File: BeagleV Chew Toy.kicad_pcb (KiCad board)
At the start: 2 copper layers, 57.2 x 51.7 mm, 147 parts, among them J1 Conn_02x05_Counter_Clockwise, J2 Conn_02x05_Counter_Clockwise, J3 Conn_02x05_Counter_Clockwise, U1 74HC245, U2 74HC245, U3 74HC245, U4 74HC245

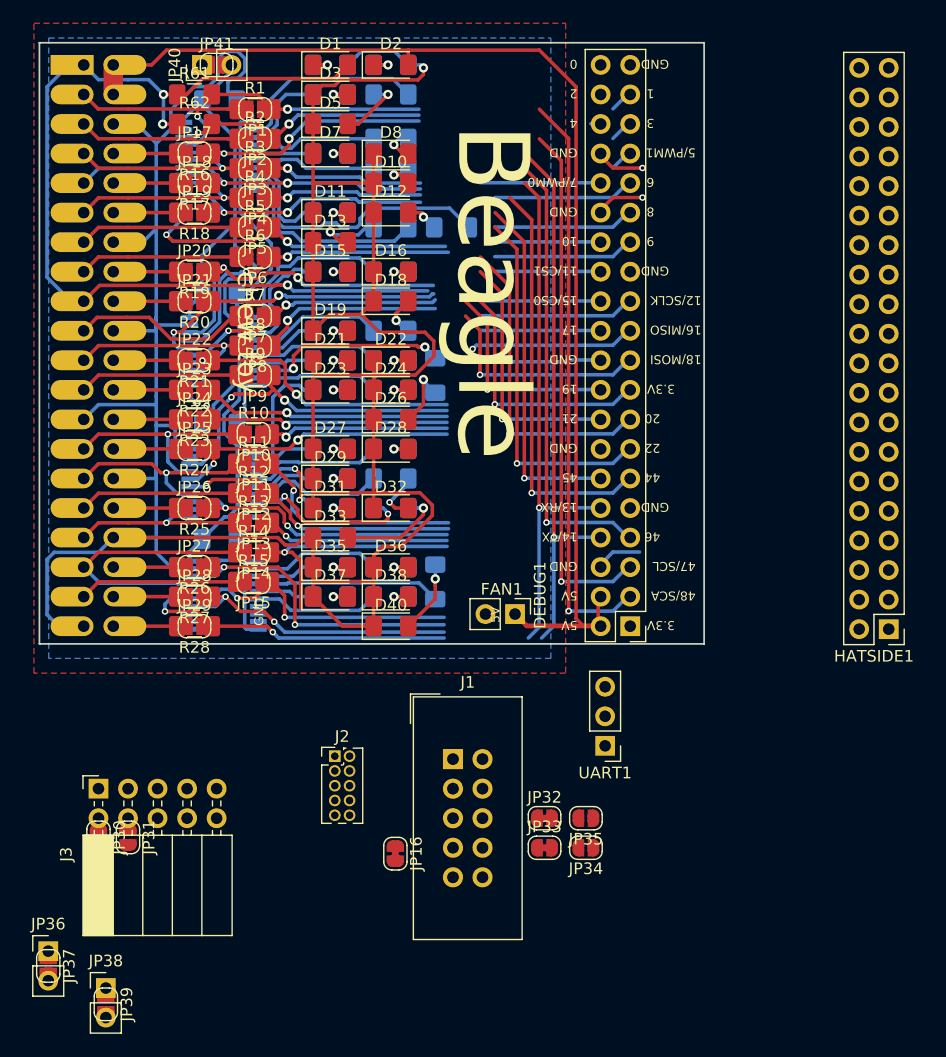
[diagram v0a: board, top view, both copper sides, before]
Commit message: main part of the PCB is done
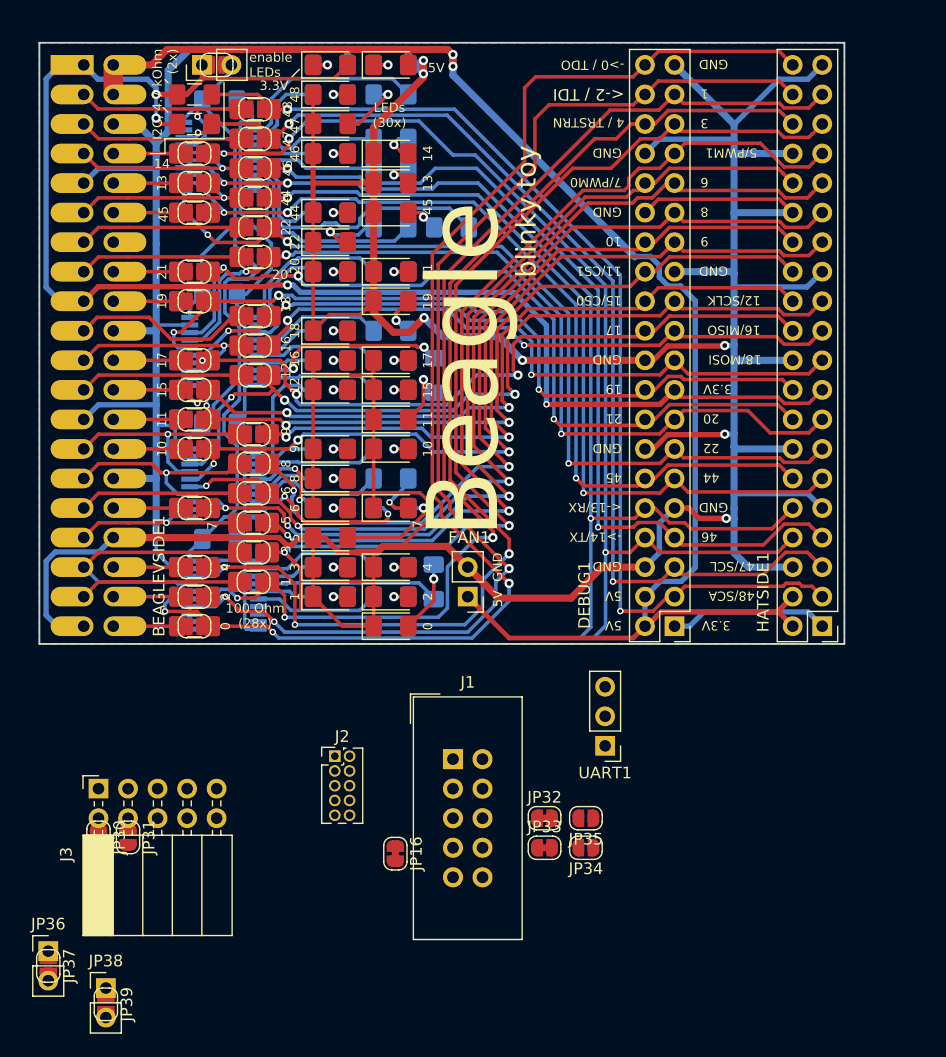
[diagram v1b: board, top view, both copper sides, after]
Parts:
- moved HATSIDE1 5.72 mm to (193.2, 129.0)
- moved FAN1 4.33 mm to (162.7, 126.5), turned to 180 degrees
- moved DEBUG1 3.81 mm to (180.5, 129.0)
- moved R32 0.13 mm to (159.8, 125.2)
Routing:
- net GND: track 359.5 -> 557.6 mm, vias 3 -> 7
- net /GPIO0_TDO_FROM_SOC: track 29.0 -> 110.9 mm, vias 2 -> 3
- net /GPIO2_TDI_TO_SOC: track 27.5 -> 105.0 mm, vias 2 -> 3
- net /GPIO1_TCK: track 27.8 -> 99.2 mm, vias 2 -> 3
- net /GPIO4_TRSTN: track 28.8 -> 99.1 mm, vias 2 -> 3
- net /GPIO3_TMS: track 23.8 -> 88.5 mm, vias 1 -> 2
- net /GPIO5/PWM: track 18.4 -> 80.5 mm, vias 1 -> 2
- net /GPIO7/PWM: track 35.1 -> 82.4 mm, vias 2 -> 3
- net /GPIO6: track 37.0 -> 83.1 mm, vias 2 -> 3
- net /GPIO8: track 31.5 -> 74.8 mm, vias 1 -> 2
- net /GPIO10: track 34.4 -> 73.8 mm, vias 2 -> 3
- net +3V3: track 106.6 -> 143.3 mm
- net /GPIO9: track 28.4 -> 64.6 mm, vias 1 -> 2
- net /GPIO11/CS1: track 35.2 -> 68.7 mm, vias 2 -> 3
- net /GPIO15/CS0: track 35.4 -> 64.5 mm, vias 2 -> 3
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- added copper zone on F.Cu, net GND
- removed copper zone on F.Cu, net +3V3
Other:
- board size 57.2 x 51.7 mm -> 69.2 x 51.7 mm
- board text added: "->0 / TDO"
- board text added: "->14/TX"
- board text added: "1 kOhm (30x)"
- board text added: "100 Ohm (28x)"
- board text added: "11"
- board text added: "12"
- board text added: "13"
- board text added: "14"
- board text added: "15"
- board text added: "16"
- board text added: "18"
- board text added: "4 / TRSTRN"
- board text added: "47"
- board text added: "48"
- board text added: "5"
- board text added: "7"
- board text added: "<-13/RX"
- board text added: "<-2 / TDI"
- board text added: "BeagleV blinky toy v1 (C) 2021 snowball based on BeagleV chew toy by John 'Warthog9' Hawley CC-BY-SA 4.0 https://github.com/BBBSnowball/beaglev-chewtoy"
- board text added: "I2C, 4.7 kOhm (2x)"
- board text added: "LEDs (30x)"
- board text added: "blinky toy"
- board text added: "enable LEDs"
- board text removed: "(C) 2021 John 'Warthog9' Hawley CC-BY-SA 4.0 https://github.com/warthog9/beaglev-chewtoy v1"
- board text removed: "13/RX"
- board text removed: "14/TX"
- board text removed: "chew toy"
